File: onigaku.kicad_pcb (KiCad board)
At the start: 2 copper layers, 351.3 x 110.2 mm, 312 parts, among them J1 MJ-4PP-9, J2 MJ-4PP-9, U1 Elite-C, U2 Elite-C

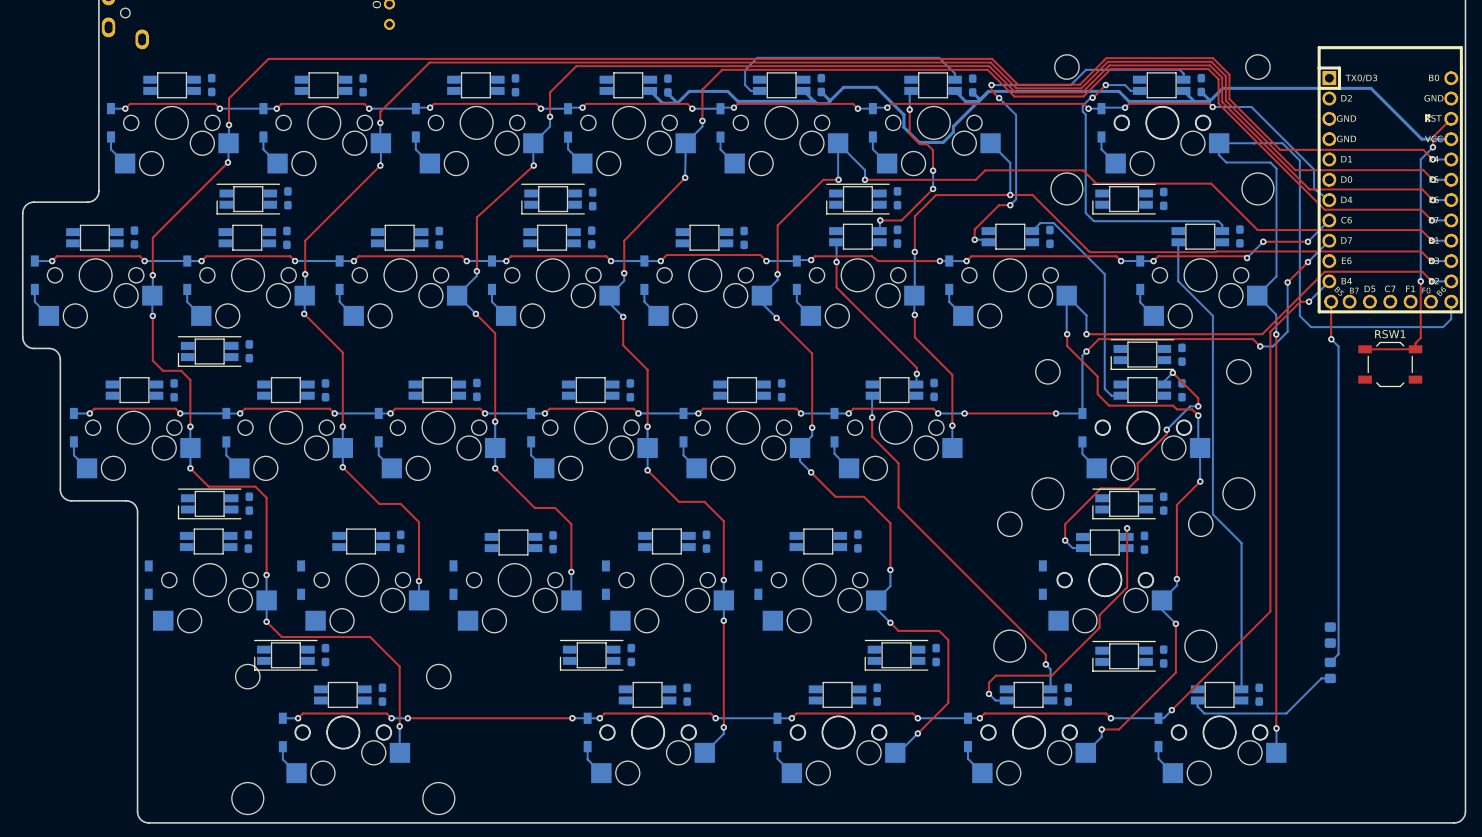
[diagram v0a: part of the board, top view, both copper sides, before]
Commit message: routing WIP
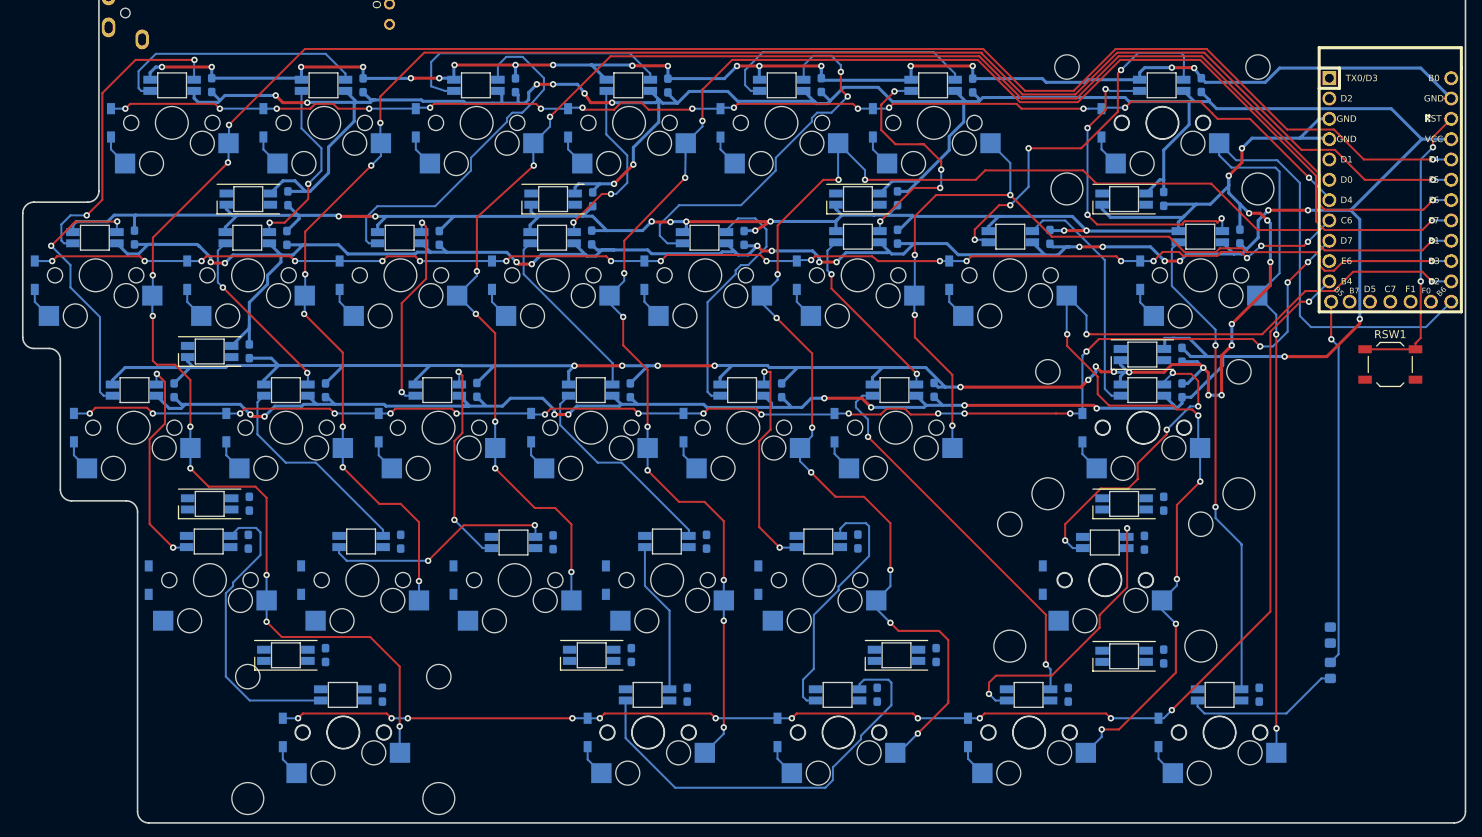
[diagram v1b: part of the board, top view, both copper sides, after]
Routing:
- net GNDA: track 0.00 -> 652.7 mm, vias 0 -> 46
- net VDD: track 129.4 -> 706.8 mm, vias 0 -> 32
- net Net-(LED79-Pad4): track 0.00 -> 53.8 mm
- net Net-(LED29-Pad2): track 0.00 -> 47.6 mm, vias 0 -> 2
- net Net-(LED27-Pad2): track 0.00 -> 45.1 mm
- net Net-(LED25-Pad2): track 0.00 -> 39.1 mm, vias 0 -> 2
- net Net-(LED66-Pad2): track 0.00 -> 37.3 mm
- net Net-(LED27-Pad4): track 0.00 -> 35.6 mm
- net Net-(LED39-Pad2): track 0.00 -> 33.4 mm, vias 0 -> 2
- net Net-(LED25-Pad4): track 0.00 -> 32.4 mm
- net Net-(LED43-Pad2): track 0.00 -> 32.1 mm
- net Net-(LED70-Pad2): track 0.00 -> 31.4 mm
- net Net-(LED57-Pad2): track 0.00 -> 29.0 mm, vias 0 -> 2
- net Net-(LED67-Pad4): track 0.00 -> 29.0 mm, vias 0 -> 2
- net Net-(LED55-Pad2): track 0.00 -> 27.4 mm, vias 0 -> 2
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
